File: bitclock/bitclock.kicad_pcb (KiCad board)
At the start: 2 copper layers, 61 x 61 mm, 11 parts, among them IC1 ATTINY13-S, P1 USB_OTG, SW1 Hour, SW2 Minute, U1 TA23-11EWA, U2 TM1637

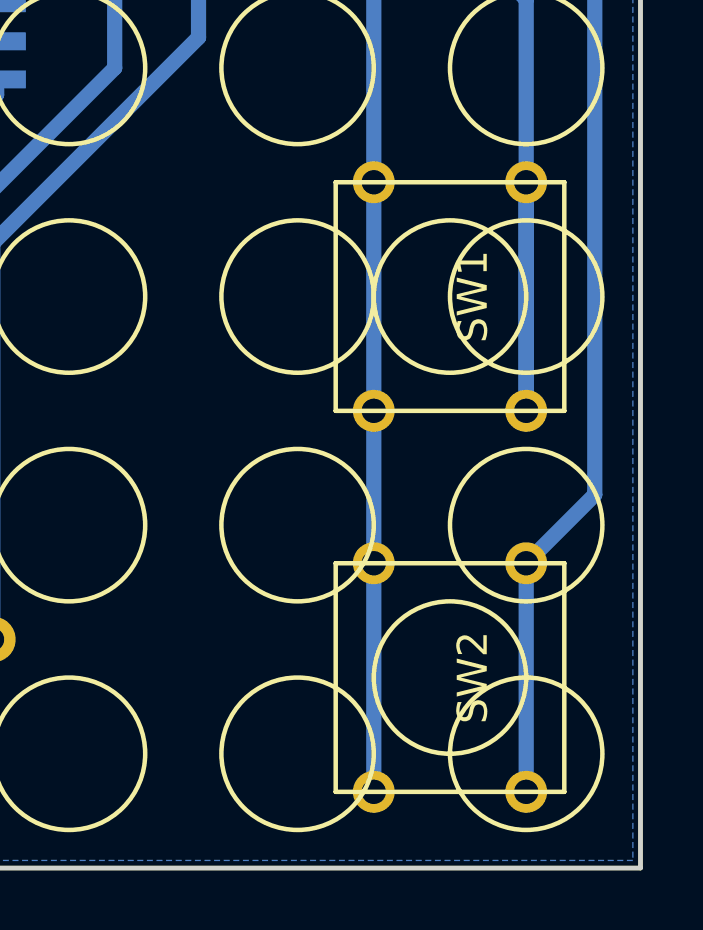
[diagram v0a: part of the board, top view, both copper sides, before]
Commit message: lora1278 breakout: added
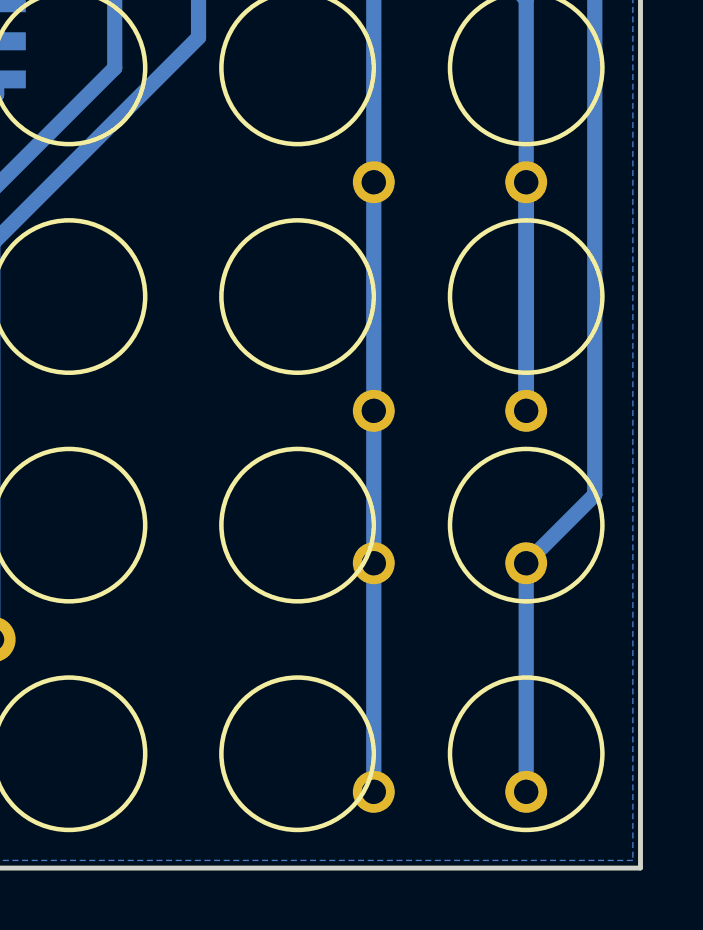
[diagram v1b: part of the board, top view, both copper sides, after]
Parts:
- SW1, SW2: moved to B.Cu
- turned SW1 to 90 degrees
- turned SW2 to 90 degrees
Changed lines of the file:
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@@
     (links 42)
     (no_connects 0)
-    (area 116.155 50.524999 178.075001 113.4843)
+    (area 116.764999 50.724999 177.875001 111.835001)
     (thickness 1.6)
     (drawings 5)
@@
     )
   )
-  (module Buttons_Switches_ThroughHole:SW_PUSH_SMALL (layer F.Cu)
-    (at 171.45 92.71 270)
-    (fp_text reference SW1 (at 0 -0.762 270) (layer F.SilkS)
-      (effects (font (size 1 1) (thickness 0.15)))
-    )
-    (fp_text value Hour (at 0 1.016 270) (layer F.Fab)
-      (effects (font (size 1 1) (thickness 0.15)))
-    )
-    (fp_circle (center 0 0) (end 0 -2.54) (layer F.SilkS) (width 0.15))
-    (fp_line (start -3.81 -3.81) (end 3.81 -3.81) (layer F.SilkS) (width 0.15))
-    (fp_line (start 3.81 -3.81) (end 3.81 3.81) (layer F.SilkS) (width 0.15))
-    (fp_line (start 3.81 3.81) (end -3.81 3.81) (layer F.SilkS) (width 0.15))
-    (fp_line (start -3.81 -3.81) (end -3.81 3.81) (layer F.SilkS) (width 0.15))
-    (pad 1 thru_hole circle (at 3.81 -2.54 270) (size 1.397 1.397) (drill 0.8128) (layers *.Cu *.Mask F.SilkS)
+  (module Buttons_Switches_ThroughHole:SW_PUSH_SMALL (layer B.Cu)
+    (at 171.45 92.71 90)
+    (fp_text reference SW1 (at 0 0.762 90) (layer B.SilkS)
+      (effects (font (size 1 1) (thickness 0.15)) (justify mirror))
+    )
+    (fp_text value Hour (at 0 -1.016 90) (layer B.Fab)
+      (effects (font (size 1 1) (thickness 0.15)) (justify mirror))
+    )
+    (fp_circle (center 0 0) (end 0 2.54) (layer B.SilkS) (width 0.15))
+    (fp_line (start -3.81 3.81) (end 3.81 3.81) (layer B.SilkS) (width 0.15))
+    (fp_line (start 3.81 3.81) (end 3.81 -3.81) (layer B.SilkS) (width 0.15))
+    (fp_line (start 3.81 -3.81) (end -3.81 -3.81) (layer B.SilkS) (width 0.15))
+    (fp_line (start -3.81 3.81) (end -3.81 -3.81) (layer B.SilkS) (width 0.15))
+    (pad 1 thru_hole circle (at 3.81 2.54 90) (size 1.397 1.397) (drill 0.8128) (layers *.Cu *.Mask B.SilkS)
       (net 12 "Net-(SW1-Pad1)"))
-    (pad 2 thru_hole circle (at 3.81 2.54 270) (size 1.397 1.397) (drill 0.8128) (layers *.Cu *.Mask F.SilkS)
+    (pad 2 thru_hole circle (at 3.81 -2.54 90) (size 1.397 1.397) (drill 0.8128) (layers *.Cu *.Mask B.SilkS)
       (net 13 SEG1))
-    (pad 1 thru_hole circle (at -3.81 -2.54 270) (size 1.397 1.397) (drill 0.8128) (layers *.Cu *.Mask F.SilkS)
+    (pad 1 thru_hole circle (at -3.81 2.54 90) (size 1.397 1.397) (drill 0.8128) (layers *.Cu *.Mask B.SilkS)
       (net 12 "Net-(SW1-Pad1)"))
-    (pad 2 thru_hole circle (at -3.81 2.54 270) (size 1.397 1.397) (drill 0.8128) (layers *.Cu *.Mask F.SilkS)
+    (pad 2 thru_hole circle (at -3.81 -2.54 90) (size 1.397 1.397) (drill 0.8128) (layers *.Cu *.Mask B.SilkS)
       (net 13 SEG1))
   )
-  (module Buttons_Switches_ThroughHole:SW_PUSH_SMALL (layer F.Cu)
-    (at 171.45 105.41 270)
-    (fp_text reference SW2 (at 0 -0.762 270) (layer F.SilkS)
-      (effects (font (size 1 1) (thickness 0.15)))
-    )
-    (fp_text value Minute (at 0 1.016 270) (layer F.Fab)
-      (effects (font (size 1 1) (thickness 0.15)))
-    )
-    (fp_circle (center 0 0) (end 0 -2.54) (layer F.SilkS) (width 0.15))
-    (fp_line (start -3.81 -3.81) (end 3.81 -3.81) (layer F.SilkS) (width 0.15))
-    (fp_line (start 3.81 -3.81) (end 3.81 3.81) (layer F.SilkS) (width 0.15))
-    (fp_line (start 3.81 3.81) (end -3.81 3.81) (layer F.SilkS) (width 0.15))
-    (fp_line (start -3.81 -3.81) (end -3.81 3.81) (layer F.SilkS) (width 0.15))
-    (pad 1 thru_hole circle (at 3.81 -2.54 270) (size 1.397 1.397) (drill 0.8128) (layers *.Cu *.Mask F.SilkS)
+  (module Buttons_Switches_ThroughHole:SW_PUSH_SMALL (layer B.Cu)
+    (at 171.45 105.41 90)
+    (fp_text reference SW2 (at 0 0.762 90) (layer B.SilkS)
+      (effects (font (size 1 1) (thickness 0.15)) (justify mirror))
+    )
+    (fp_text value Minute (at 0 -1.016 90) (layer B.Fab)
+      (effects (font (size 1 1) (thickness 0.15)) (justify mirror))
+    )
+    (fp_circle (center 0 0) (end 0 2.54) (layer B.SilkS) (width 0.15))
+    (fp_line (start -3.81 3.81) (end 3.81 3.81) (layer B.SilkS) (width 0.15))
+    (fp_line (start 3.81 3.81) (end 3.81 -3.81) (layer B.SilkS) (width 0.15))
+    (fp_line (start 3.81 -3.81) (end -3.81 -3.81) (layer B.SilkS) (width 0.15))
+    (fp_line (start -3.81 3.81) (end -3.81 -3.81) (layer B.SilkS) (width 0.15))
+    (pad 1 thru_hole circle (at 3.81 2.54 90) (size 1.397 1.397) (drill 0.8128) (layers *.Cu *.Mask B.SilkS)
       (net 14 "Net-(SW2-Pad1)"))
-    (pad 2 thru_hole circle (at 3.81 2.54 270) (size 1.397 1.397) (drill 0.8128) (layers *.Cu *.Mask F.SilkS)
+    (pad 2 thru_hole circle (at 3.81 -2.54 90) (size 1.397 1.397) (drill 0.8128) (layers *.Cu *.Mask B.SilkS)
       (net 13 SEG1))
-    (pad 1 thru_hole circle (at -3.81 -2.54 270) (size 1.397 1.397) (drill 0.8128) (layers *.Cu *.Mask F.SilkS)
+    (pad 1 thru_hole circle (at -3.81 2.54 90) (size 1.397 1.397) (drill 0.8128) (layers *.Cu *.Mask B.SilkS)
       (net 14 "Net-(SW2-Pad1)"))
-    (pad 2 thru_hole circle (at -3.81 2.54 270) (size 1.397 1.397) (drill 0.8128) (layers *.Cu *.Mask F.SilkS)
+    (pad 2 thru_hole circle (at -3.81 -2.54 90) (size 1.397 1.397) (drill 0.8128) (layers *.Cu *.Mask B.SilkS)
       (net 13 SEG1))
   )
